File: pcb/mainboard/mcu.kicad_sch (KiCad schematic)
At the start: 23 parts, among them J5 SM03B-SRSS-TB, SW1 SW, SW2 SW, U13 W25Q32JV, U14 RP2040, Y2 12MHz

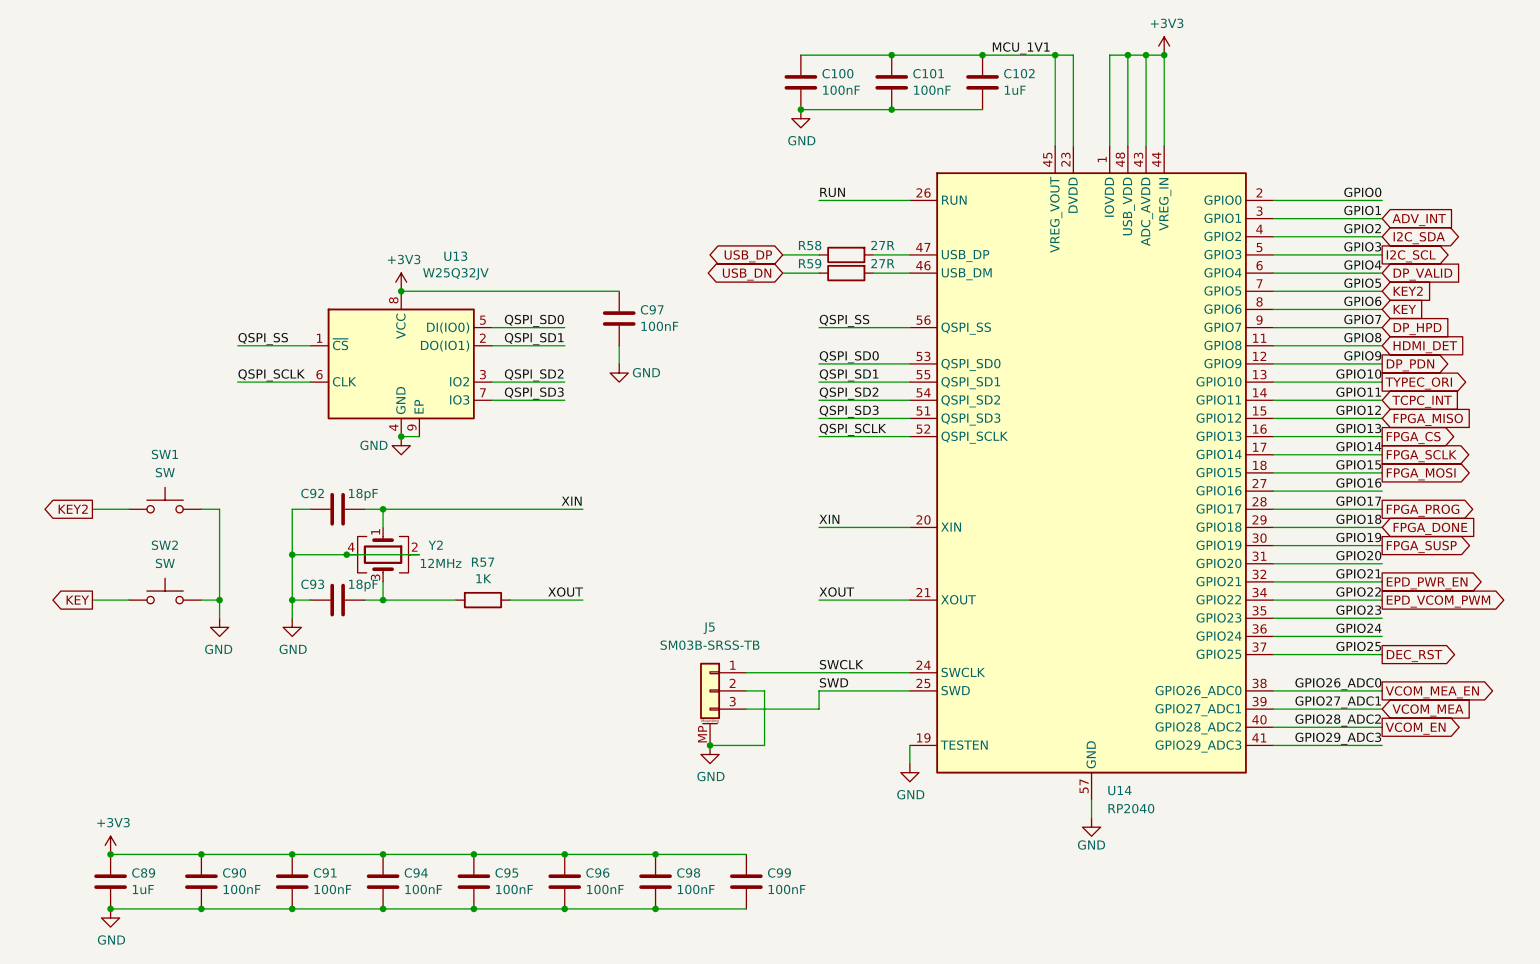
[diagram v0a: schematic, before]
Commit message: Bug fixes and changes for r0p8
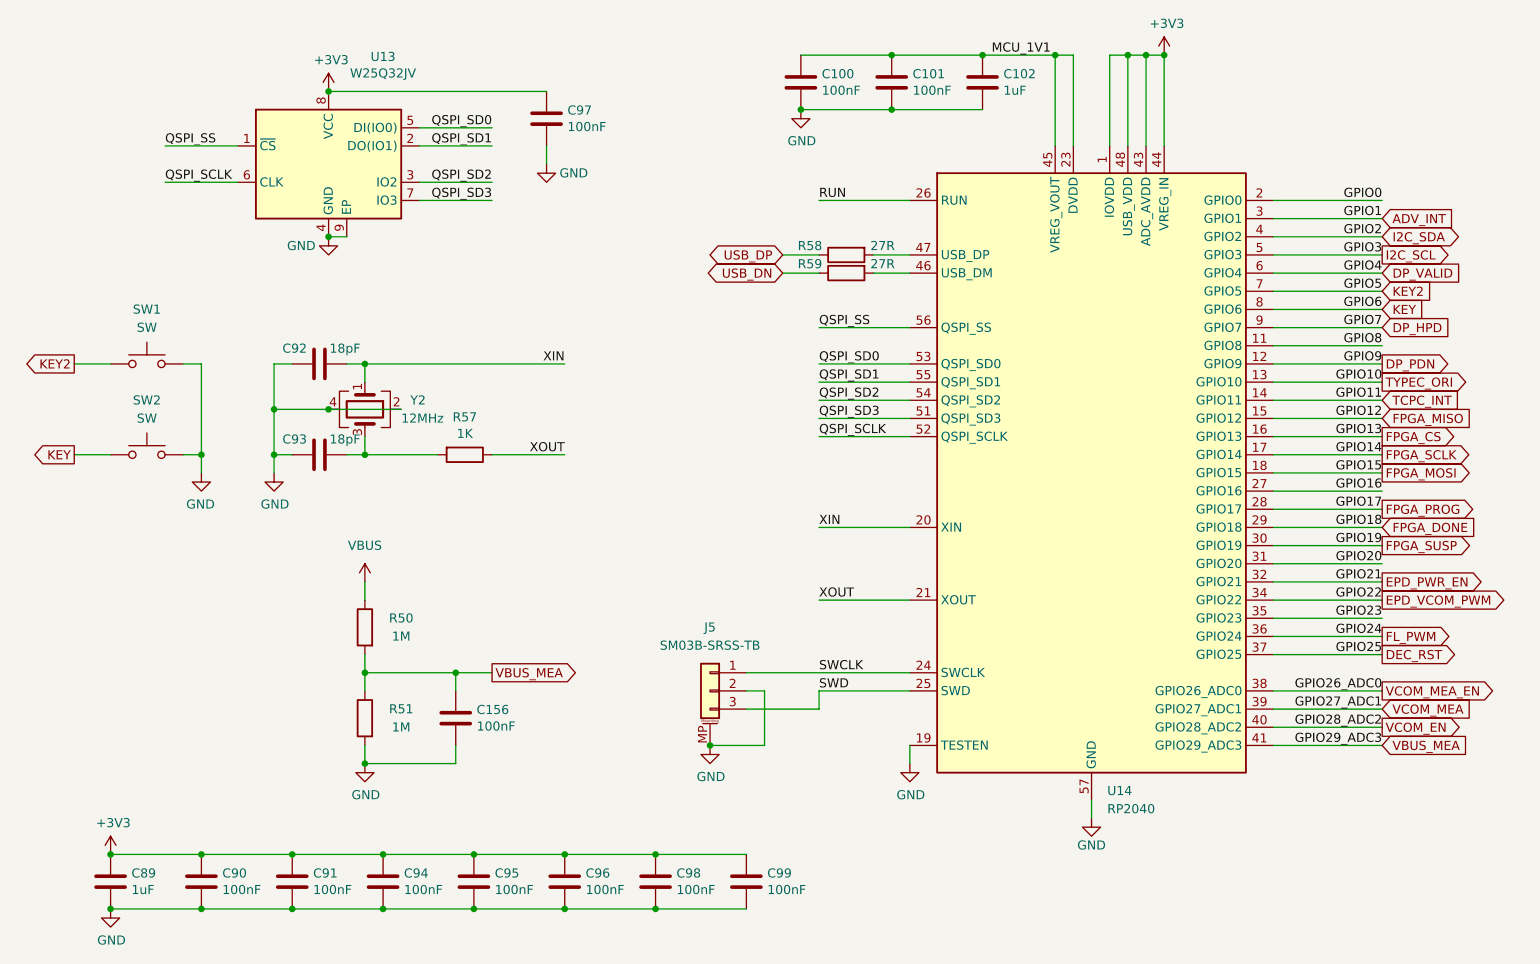
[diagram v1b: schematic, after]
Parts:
- added C156: 100nF, Capacitor_SMD:C_0402_1005Metric, symbol Device:C
- added R50, R51: 1M, Resistor_SMD:R_0402_1005Metric, symbol Device:R
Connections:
- net GND: now also C156.2, R51.2
- net GPIO24 renamed FL_PWM
- net GPIO29_ADC3 renamed VBUS_MEA
- net VBUS_MEA: now also C156.1, R50.2, R51.1
- net HDMI_DET renamed GPIO8
- new net VBUS: R50.1
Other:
- company: Copyright 2022 Modos / Engineer: Wenting Zhang -> Copyright 2024 Wenting Zhang
- title: Caster EPDC -> Glider
- moved on the sheet: C92, C93, C97, R57, SW1, SW2, U13, Y2

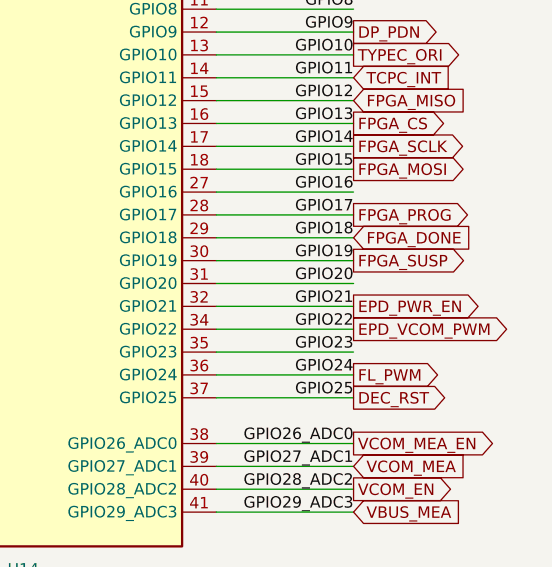
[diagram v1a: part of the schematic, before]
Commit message: PCB r0p8
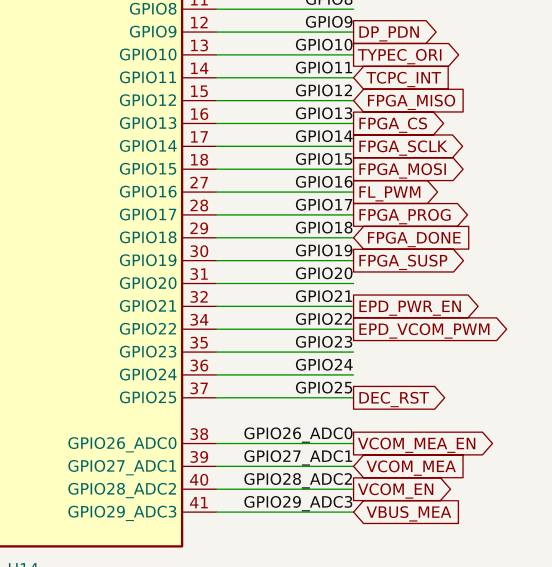
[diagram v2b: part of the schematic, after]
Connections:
- net GPIO16 is gone; now on net FL_PWM: U14.27 (GPIO16)
- net FL_PWM: no longer U14.36 (GPIO24)
- new net GPIO24: U14.36 (GPIO24)
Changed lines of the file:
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@@
 	(global_label "FL_PWM"
 		(shape output)
-		(at 233.68 124.46 0)
+		(at 233.68 104.14 0)
 		(effects
 			(font
@@
 		)
 		(property "Intersheetrefs" "${INTERSHEET_REFS}"
-			(at 337.82 238.76 0)
+			(at 337.82 218.44 0)
 			(effects
 				(font

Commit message: BOM adjustments
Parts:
- U13: LCSC C571260 -> (none)
- Y2: footprint Oscillator:Oscillator_SMD_Abracon_ASE-4Pin_3.2x2.5mm -> Crystal:Crystal_SMD_3225-4Pin_3.2x2.5mm
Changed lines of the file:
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@@
 			)
 		)
-		(property "LCSC" "C571260"
+		(property "LCSC" ""
 			(at 86.36 58.42 0)
 			(effects
@@
 			)
 		)
-		(property "Footprint" "Oscillator:Oscillator_SMD_Abracon_ASE-4Pin_3.2x2.5mm"
+		(property "Footprint" "Crystal:Crystal_SMD_3225-4Pin_3.2x2.5mm"
 			(at 91.44 92.71 0)
 			(effects
